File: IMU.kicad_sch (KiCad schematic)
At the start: 1 part, among them U2 4754

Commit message: C14 y C1,C2,... modificados
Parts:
- U2: MANUFACTURER Adafruit -> (none); Manufacturer (none) -> Adafruit
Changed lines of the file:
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@@
 			)
 		)
-		(property "MANUFACTURER" "Adafruit"
+		(property "Manufacturer" "Adafruit"
 			(at 164.592 137.414 0)
 			(hide yes)
@@
 			)
 		)
+		(property "Field7" ""
+			(at 165.1 107.95 0)
+			(hide yes)
+			(show_name no)
+			(do_not_autoplace no)
+			(effects
+				(font
+					(size 1.27 1.27)
+				)
+			)
+		)

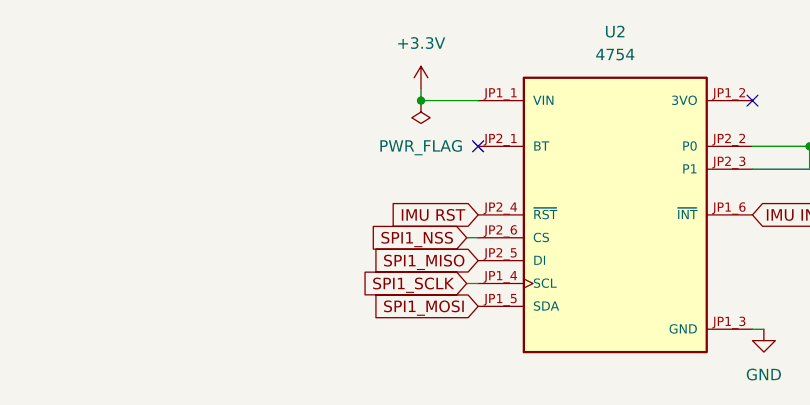
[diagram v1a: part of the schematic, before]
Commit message: Avance 02/08
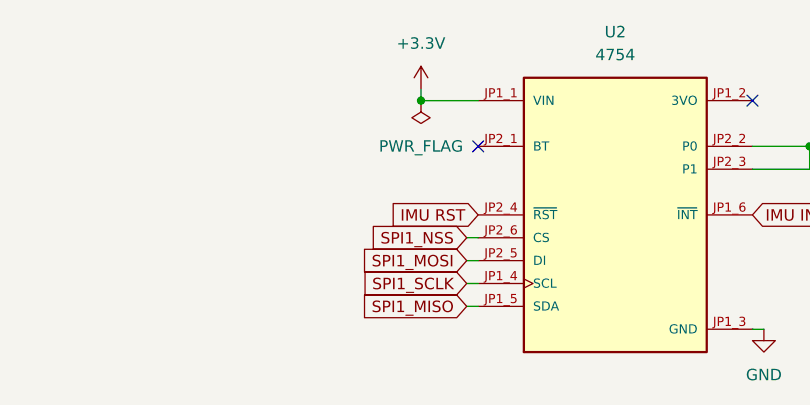
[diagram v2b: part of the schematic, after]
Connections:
- net SPI1_MISO: now also U2.JP1_5 (SDA); no longer U2.JP2_5 (DI)
- net SPI1_MOSI: now also U2.JP2_5 (DI); no longer U2.JP1_5 (SDA)
